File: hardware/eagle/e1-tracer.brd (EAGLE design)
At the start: 160 x 120 mm, 108 parts, among them IC1 W25Q80DVSNIG, IC2 MCP1703T-1202E/CB, IC3 TPS73633DCQR, IC4 ASEM1-12.000MHZ-LC-T, J1 PASSTHROUGH, M1 MENTOR_12701001, M2 MENTOR_12701001, T1 BC847C, T2 BC847C, U1 ICE40UP5K-SG48I, U2 IP4234CZ6, U3 IDT82V2081, U4 IDT82V2081, U5 2.048 Mhz, U6 1.544 MHz, X1 MINI-USB-SHIELD-UX60-MB-5ST

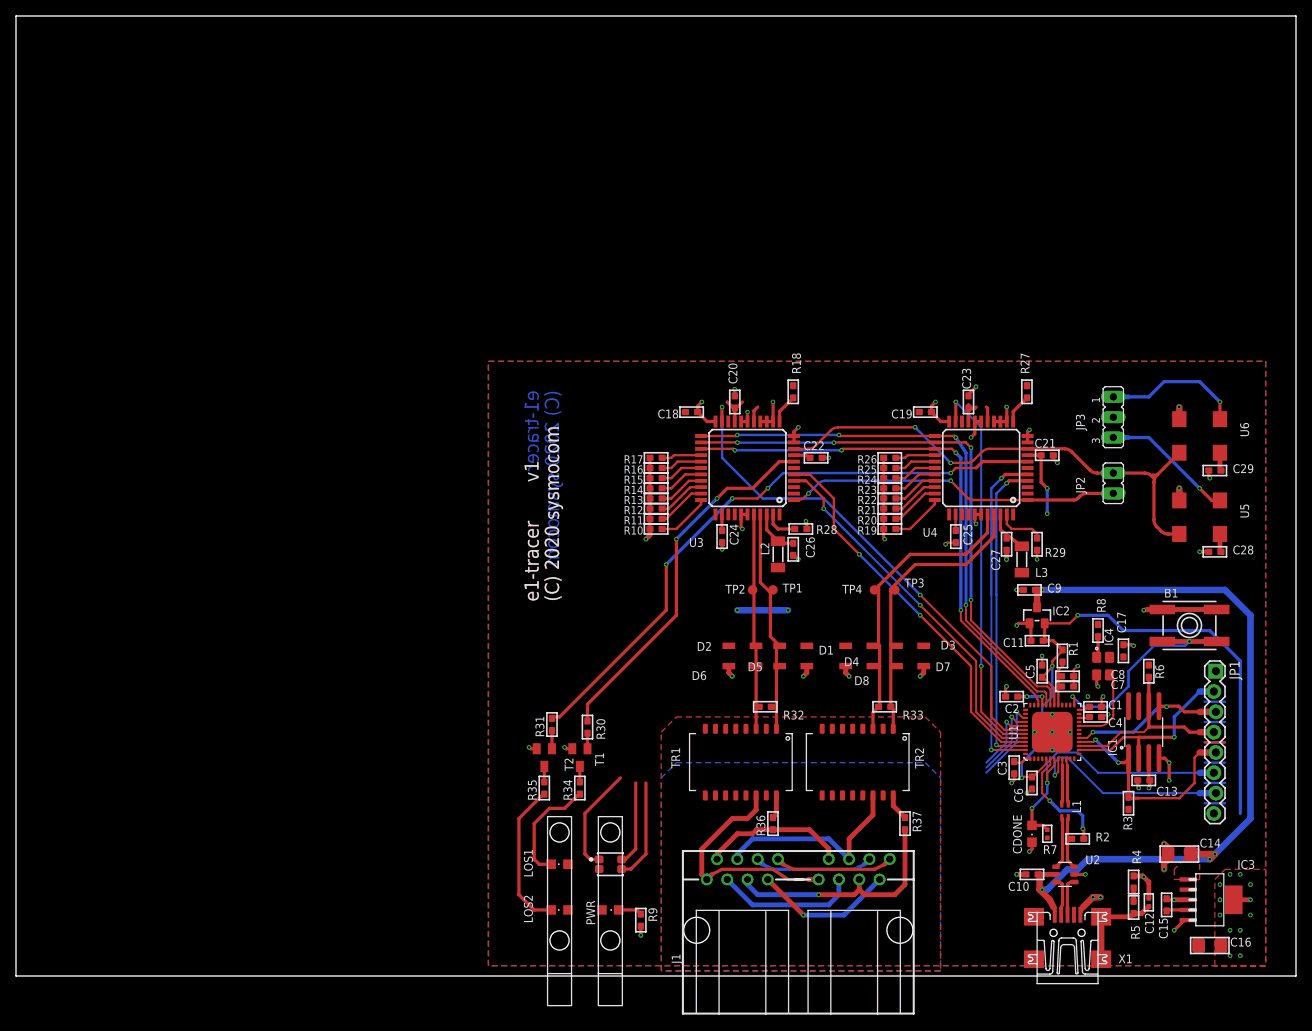
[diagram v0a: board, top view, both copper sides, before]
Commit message: e1-tracer: finish PCB
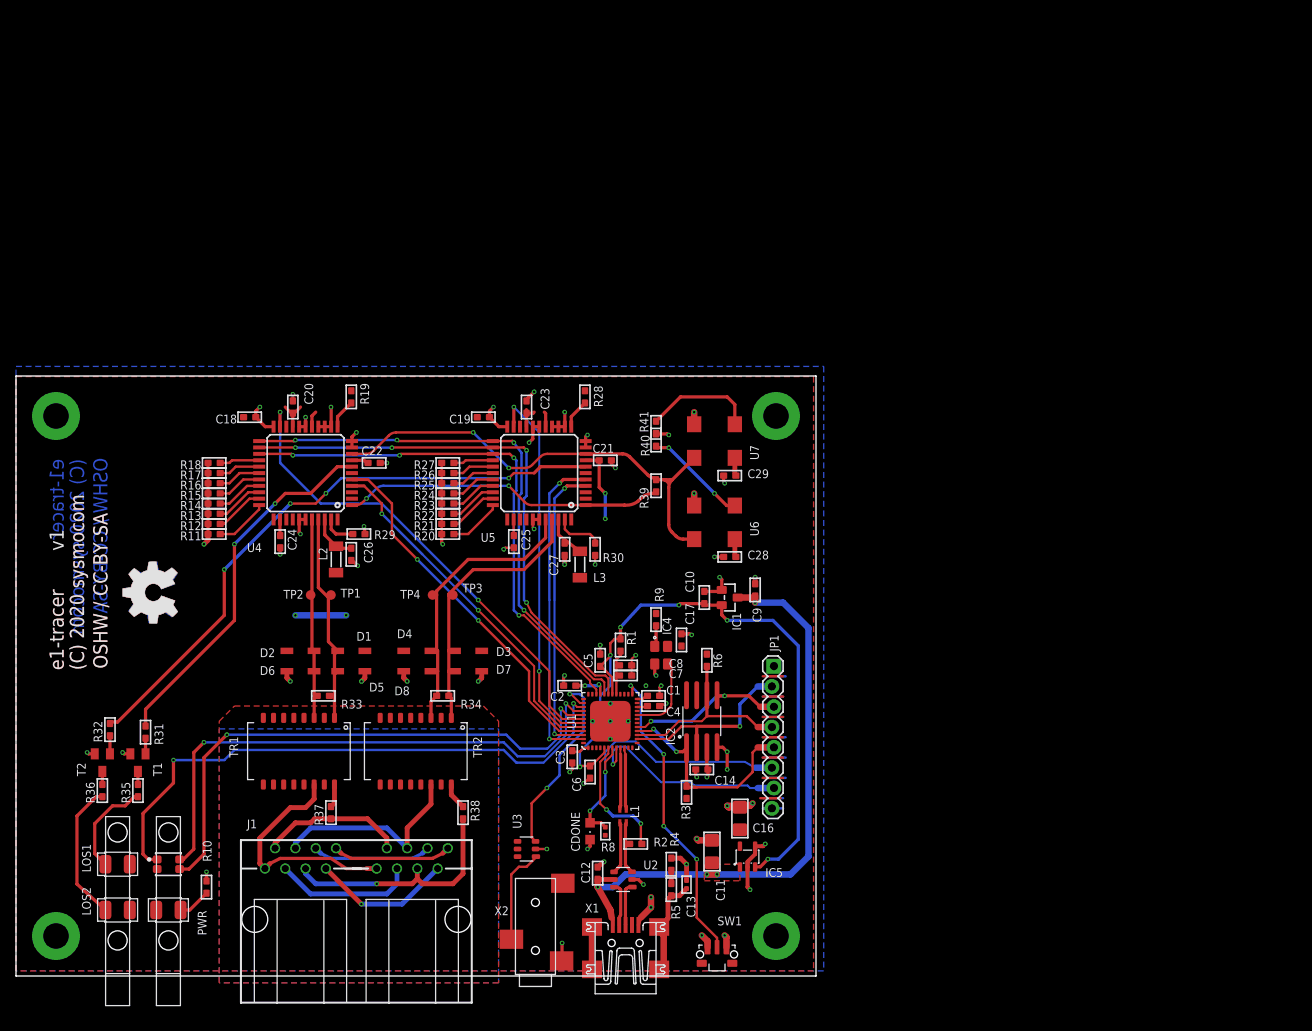
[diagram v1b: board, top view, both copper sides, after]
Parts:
- removed B1: (no value), microbuilder:EVQ-Q2
- removed C15: 10n, rc-sysmocom:_0603@1
- removed IC3: TPS73633DCQR, laforge:SOT223-6
- removed JP2: TCLK/MCLK, jumper:JP1
- removed JP3: 1544/2048, jumper:JP2
- removed R7: 2.2k, rc-sysmocom:_0402
- added IC5: TLV70233DBVR, tlv700xx:SOT23-DBV
- added R38: 1k, rc-sysmocom:_0603
- added R39, R40, R41: DNP, rc-sysmocom:_0603
- added SW1: TACTSW-TL3340, tact-switches:TL3340-ORIG
- added U$1, U$3: (no value), oshw:OSHW_8MM_COPPER
- added U7: 1.544 MHz, laforge:HC73
- added X2: JACK2.5_SJ-2523, laforge:JACK2.5_SJ-2523
- C11: value 1u -> 22u; device rc-sysmocom:_0603@1 -> rc-sysmocom:1206@1
- C12: value 10n -> 1u; device rc-sysmocom:_0402@1 -> rc-sysmocom:_0603@1
- C13: value 100n -> 10n; device rc-sysmocom:_0603@1 -> rc-sysmocom:_0402@1
- C14: value 22u -> 100n; device rc-sysmocom:1206@1 -> rc-sysmocom:_0603@1
- IC1: value W25Q80DVSNIG -> MCP1703T-1202E/CB; device spiflash:SO08COMBINED -> MCP170x:SOT23-3
- IC2: value MCP1703T-1202E/CB -> W25Q80DVSNIG; device MCP170x:SOT23-3 -> spiflash:SO08COMBINED
- LOS1, LOS2: value RED -> LEDPLCC2-MIN-red; device led:CHIPLED_0805 -> LED-PLCC2:PLCC2-MIN
- PWR: value GREEN -> LEDPLCC2-MIN-green; device led:CHIPLED_0805 -> LED-PLCC2:PLCC2-MIN
- R10: value 10k -> 68
- R28: value 3k 1% -> 10k
- R30: value 10k -> 3k 1%
- R32: value 120 -> 10k
- R34: value 68 -> 120
- R35: value 68 -> 330
- R36: value 1k -> 330
- R8: value 10k -> 2.2k; device rc-sysmocom:_0603 -> rc-sysmocom:_0402
- R9: value 68 -> 10k
- U3: value IDT82V2081 -> IP4234CZ6; device laforge:TQFP44 -> laforge:TSOP-6
- U5: value 2.048 Mhz -> IDT82V2081; device laforge:HC73 -> laforge:TQFP44
- U6: value 1.544 MHz -> 2.048 Mhz
- moved U5 85.4 mm to (65.4, 62.9)
- moved R29 84.8 mm to (42.9, 55.2), turned to 180 degrees
- moved U4 84.5 mm to (36.2, 62.9)
- moved R36 83.9 mm to (10.8, 23.2)
- moved R32 82.0 mm to (11.7, 30.8), turned to 90 degrees
- moved R18 72.9 mm to (24.8, 64.1), turned to 180 degrees
- moved R27 72.9 mm to (54.0, 64.1), turned to 180 degrees
- moved R10 71.8 mm to (23.8, 11.1), turned to 90 degrees
- moved R37 71.8 mm to (39.4, 20.4)
- moved R33 70.2 mm to (38.4, 35.0)
- moved R19 69.3 mm to (41.9, 72.4), turned to 90 degrees
- moved C12 69.0 mm to (72.7, 12.9)
- moved R8 66.5 mm to (73.7, 18.1)
- moved U6 61.6 mm to (89.9, 54.6)
- moved C16 60.8 mm to (90.5, 19.7), turned to 90 degrees
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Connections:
- removed net N$4 (its old number): R28.2, U3.43
- new net N$1: R30.2, U5.43
- new net UART_TX0: U3.1, X2.3
- new net VDD: U3.5
- net BOOT_SW: now also SW1.2; no longer B1.A, B1.A'
- net CDONE: now also R8.2; no longer R7.2
- net GND: now also IC1.1, IC2.4, IC5.2, IC5.4, R18.2, R27.2, R30.1, R40.2, R41.1, SW1.1, SW1.3, U3.2, U5.10, U5.11, U5.13, U5.14, U5.15, U5.17, U5.18, U5.22, U5.38, U5.39, U7.P$2, X2.1; no longer B1.B, B1.B', C15.2, IC1.4, IC2.1, IC3.3, IC3.6, JP3.2, R19.2, R28.1, R9.2, U3.10, U3.11, U3.13, U3.14, U3.15, U3.17, U3.18, U3.22, U3.38, U3.39, U5.P$2
- net IOB_32A_SPI_SO: now also IC2.2; no longer IC1.2
- net IOB_33B_SPI_SI: now also IC2.5; no longer IC1.5
- net IOB_34A_SPI_SCK: now also IC2.6; no longer IC1.6
- net IOB_35B_SPI_SS: now also IC2.1; no longer IC1.1
- net IO_A0: now also U5.24; no longer U3.24
- net IO_A1: now also U5.23; no longer U3.23
- net IO_A2: now also U5.25; no longer U3.25
- net IO_A3: now also U3.3
- net IO_A4: now also U4.21; no longer U3.21
- net IO_A5: now also U5.21; no longer U4.21
- net IO_B0: now also U4.4; no longer U3.4
- net IO_B1: now also U4.5; no longer U3.5
- net IO_B2: now also U5.4; no longer U4.4
- net IO_B3: now also U5.5; no longer U4.5
- net LOS0: now also R31.2, U4.7; no longer R30.2, U3.7
- net LOS1: now also R32.2, U5.7; no longer R31.2, U4.7
- net MCLK: now also R39.2, U5.9, U7.P$3; no longer JP2.1, U3.9, U5.P$3
- net N$10: now also R13.1, U4.31; no longer R12.1, U3.31
- net N$11: now also R14.1, U4.30; no longer R13.1, U3.30
- net N$12: now also R15.1, U4.29; no longer R14.1, U3.29
- net N$13: now also R16.1, U4.28; no longer R15.1, U3.28
- net N$14: now also R17.1, U4.27; no longer R16.1, U3.27
- net N$15: now also R22.1, U5.31; no longer R21.1, U4.31
- net N$16: now also R23.1, U5.30; no longer R22.1, U4.30
- net N$17: now also R19.1, U4.12; no longer R18.1, U3.12
- net N$18: now also R18.1, U4.26; no longer R17.1, U3.26
- net N$19: now also R24.1, U5.29; no longer R23.1, U4.29
- net N$2: now also R28.1, U5.12; no longer R27.1, U4.12
- net N$20: now also R25.1, U5.28; no longer R24.1, U4.28
- net N$21: now also R26.1, U5.27; no longer R25.1, U4.27
- net N$22: now also R27.1, U5.26; no longer R26.1, U4.26
- net N$23: now also U4.42; no longer U3.42
- net N$25: now also R9.1; no longer R8.1
- net N$26: now also R31.1; no longer R30.1
- net N$27: now also LOS1.K, R35.1; no longer LOS1.C, R34.1
- net N$28: now also R35.2; no longer R34.2
- net N$29: now also PWR.K, R10.1; no longer PWR.C, R9.1
- net N$3: now also U5.42; no longer U4.42
- net N$30: now also R37.1; no longer R36.1
- net N$31: now also R32.1; no longer R31.1
- net N$35: now also R40.1, U6.P$1; no longer JP3.3, U5.P$1
- net N$36: now also X1.M2, X1.M3; no longer C15.1, IC3.4
- net N$37: now also LOS2.K, R36.1; no longer LOS2.C, R35.1
- net N$38: now also R41.2, U7.P$1; no longer JP3.1, U6.P$1
- net N$39: now also R36.2; no longer R35.2
- net N$41: now also R38.1; no longer R37.1
- net N$42: now also R37.2; no longer R36.2
- net N$5: now also R38.2; no longer R37.2
- net N$6: now also R20.1, U5.33; no longer R19.1, U4.33
- net N$61: now also C13.1; no longer C12.1
- net N$7: now also R21.1, U5.32; no longer R20.1, U4.32
- net N$8: now also R11.1, U4.33; no longer R10.1, U3.33
- net N$9: now also R12.1, U4.32; no longer R11.1, U3.32
- net RRING: now also R33.1, U4.40; no longer R32.1, U3.40
- net RRING1: now also R34.1, U5.40; no longer R33.1, U4.40
- net RTIP: now also R33.2, U4.41; no longer R32.2, U3.41
- net RTIP1: now also R34.2, U5.41; no longer R33.2, U4.41
- net TCLK: now also R39.1, U5.1; no longer JP2.2, U3.1
- net VBUS: now also C11.1, C12.1, IC1.3, IC5.1; no longer C10.1, C14.1, IC2.3, IC3.1
- net VCC_1V2: now also C10.1, IC1.2, IC5.3; no longer C11.1, IC2.2, IC3.5
- net VCC_3V3: now also C14.1, IC2.3, IC2.7, IC2.8, IC5.5, R19.2, R28.2, R8.1, R9.2, U5.16, U5.19, U5.35, U5.8, U7.P$4; no longer C13.1, IC1.3, IC1.7, IC1.8, IC3.2, R18.2, R27.2, R7.1, R8.2, U3.16, U3.19, U3.35, U3.8, U5.P$4
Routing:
- net N$64: track 20.2 -> 69.8 mm, vias 1 -> 2
- net N$63: track 24.0 -> 73.2 mm, vias 1 -> 2
- net N$65: track 21.4 -> 69.6 mm, vias 1 -> 2
- net IO_A3: track 0.00 -> 25.0 mm, vias 0 -> 2
- net VBUS: track 98.7 -> 78.3 mm
- net VCC_3V3: track 54.0 -> 69.6 mm
- net GND: track 142.1 -> 155.0 mm, vias 74 -> 72
- net UART_TX0: track 0.00 -> 12.2 mm
- net BOOT_SW: track 27.6 -> 38.3 mm, vias 2 -> 4
- net N$1: track 0.00 -> 6.02 mm
- net VCC_1V2: track 82.4 -> 87.9 mm, vias 4 -> 6
- net MCLK: track 64.0 -> 59.0 mm
- net N$4 (its old number): track 4.17 -> 0.00 mm
- net N$35: track 16.6 -> 12.9 mm, vias 1 -> 2
- net N$38: track 17.3 -> 14.0 mm, vias 1 -> 0
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- removed copper zone on layer 1, net GND
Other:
- board size 160 x 120 mm -> 100 x 75 mm
- board text added: "OSHW / CC-BY-SA"
